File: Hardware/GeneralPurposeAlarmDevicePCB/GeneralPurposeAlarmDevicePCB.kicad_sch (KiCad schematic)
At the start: 55 parts, among them J101 Barrel_Jack_Switch_SMT, J102 0.100_2Pin, J103 0.100_2Pin, J105 S04B-XASK-1(LF)(SN)Rev2, U101 LM7805_TO220, U102 PI_ATMEGA328P-AU-InOrder

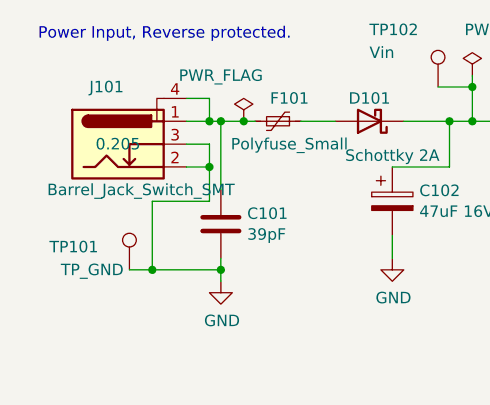
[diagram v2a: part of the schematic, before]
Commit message: Update the part number for the buzzer to a DigiKey part. This schematic is now saved in KiCAD 7.
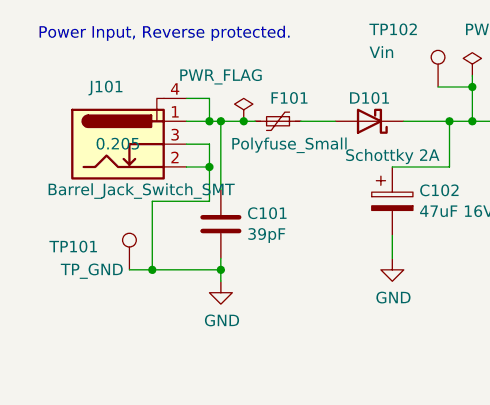
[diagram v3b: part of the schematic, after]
